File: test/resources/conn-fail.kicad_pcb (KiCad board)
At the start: 2 copper layers, 26 x 18 mm, 6 parts, among them J1 IN, J2 OUT, J3 POGO, J4 Molex

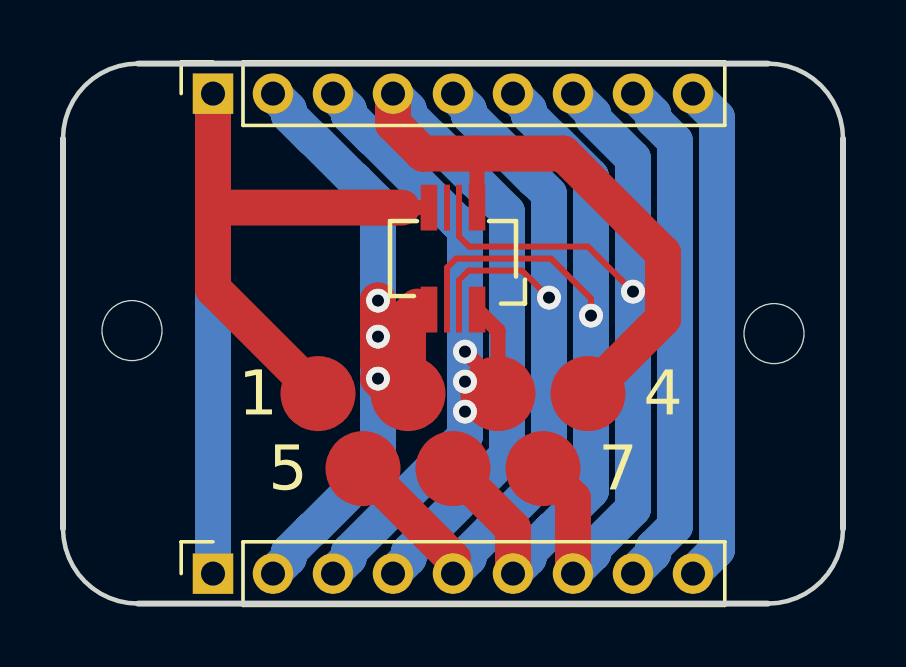
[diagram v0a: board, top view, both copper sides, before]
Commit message: Update test files to v9
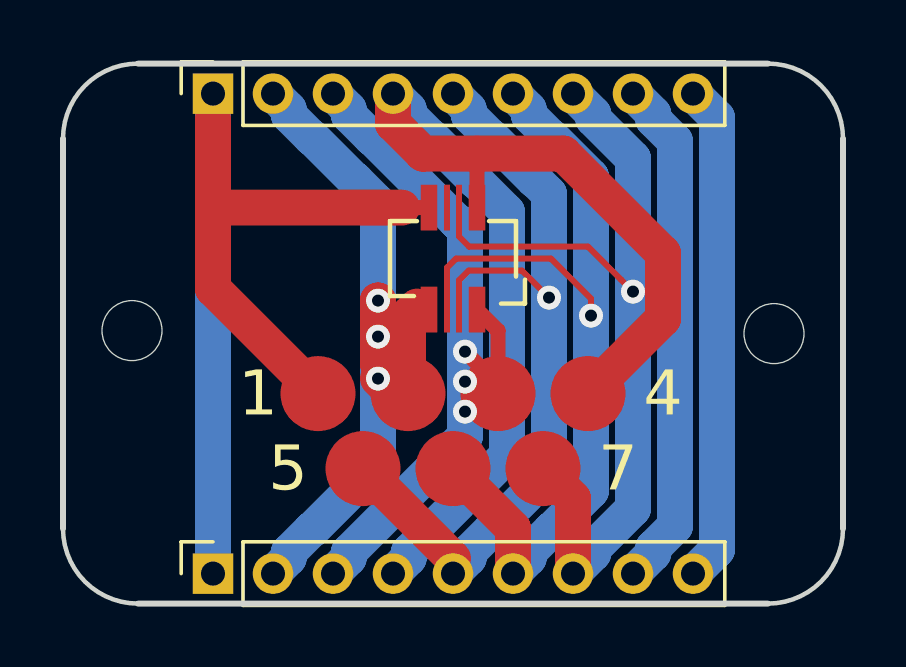
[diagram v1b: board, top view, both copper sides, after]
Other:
- net class Default removed
